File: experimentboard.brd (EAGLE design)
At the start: 105.4 x 100 mm, 72 parts, among them IC1 TL072P, IC2 LM317, IC3 LM337, Q1 27 MHz, U1 PCM1690, U2 PLL1706

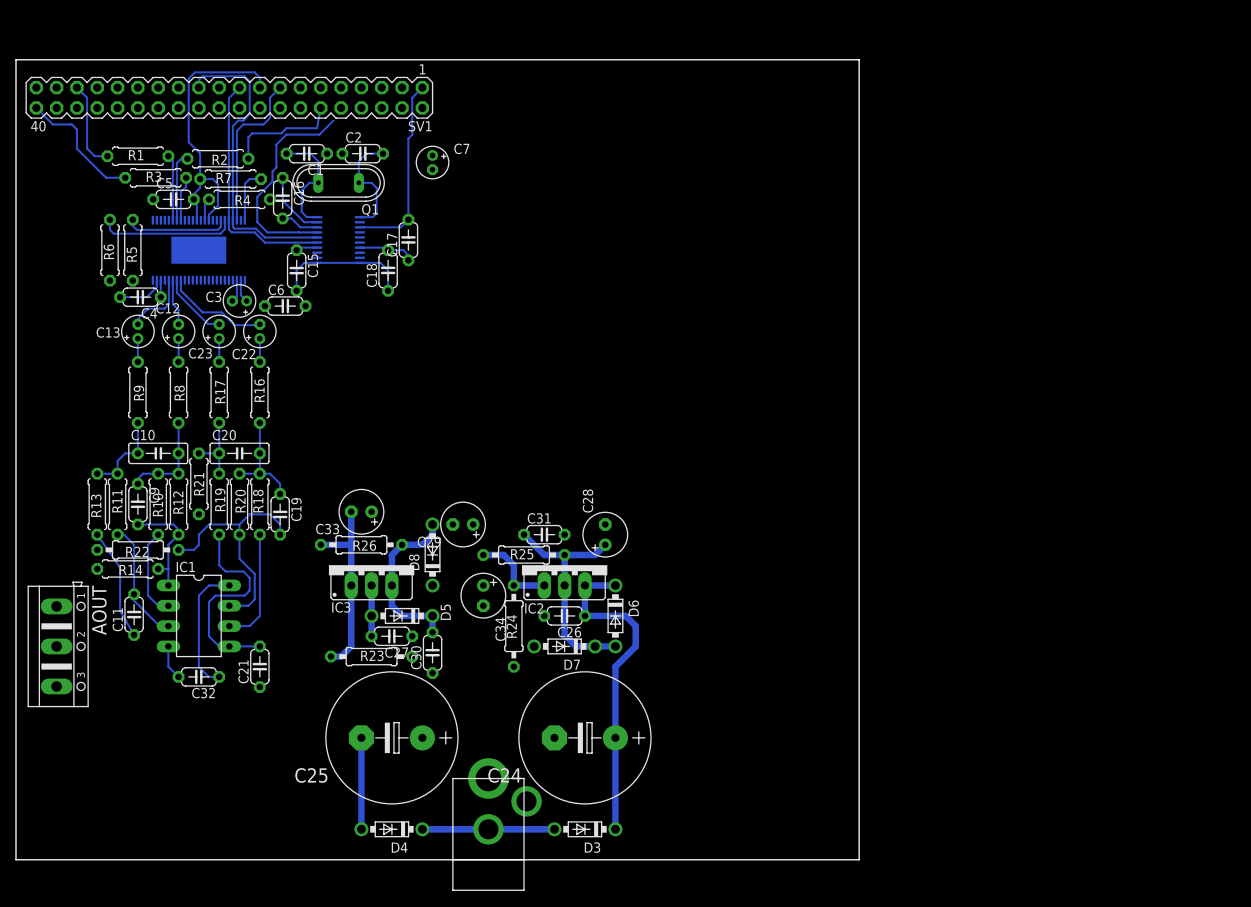
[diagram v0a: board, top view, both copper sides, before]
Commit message: Taking the Beaglebone approach
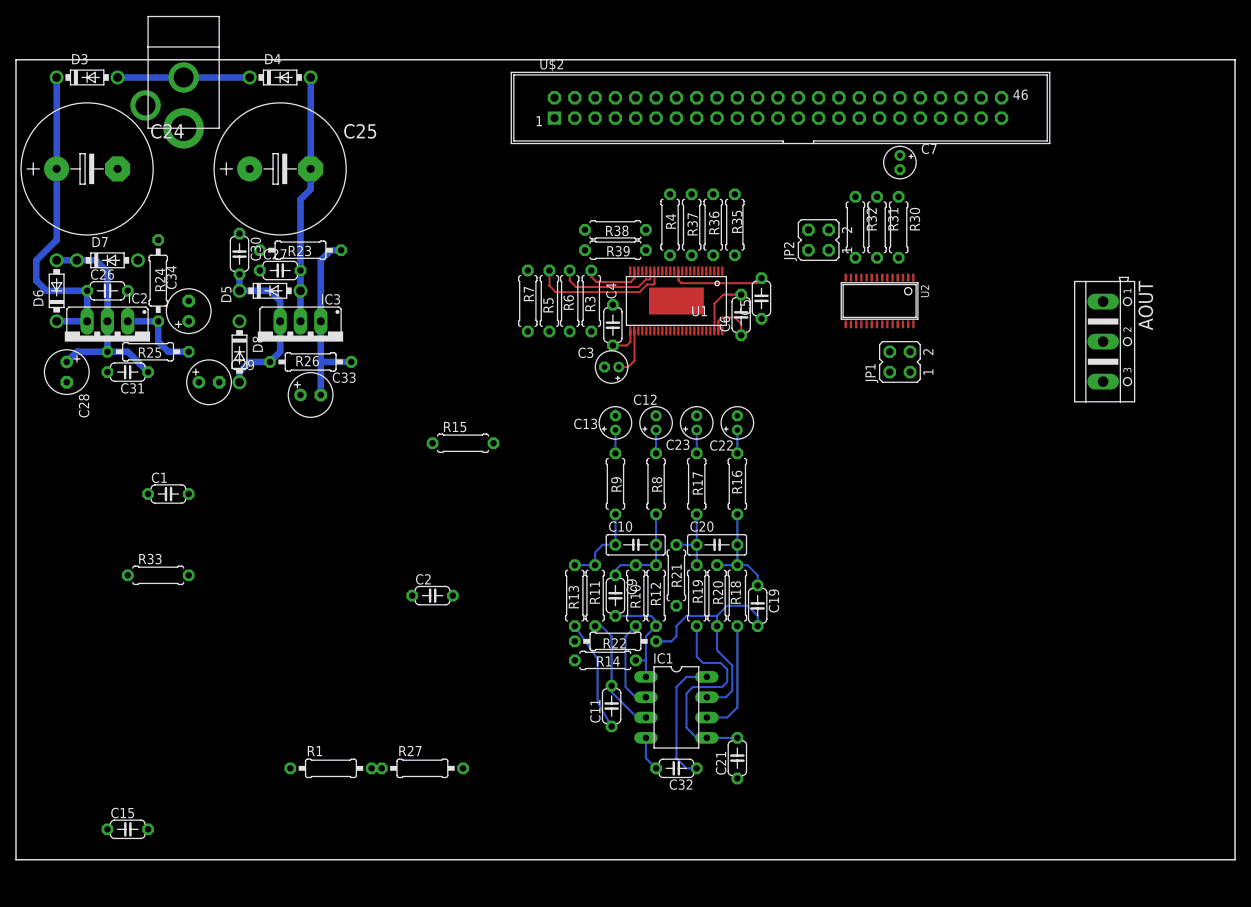
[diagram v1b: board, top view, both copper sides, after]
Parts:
- removed C16, C17, C18: 100 nF ml, rcl:C050-024X044
- removed Q1: 27 MHz, special:QS
- removed R2: 22, rcl:0207/7
- removed SV1: (no value), 0000halfgaar:MA20-2
- added JP1, JP2: (no value), jumper:JP2Q
- added R15: 680, rcl:0207/7
- added R27: 0, rcl:0207/10
- added R30, R31, R32, R33, R35, R36, R37: 22, rcl:0207/7
- added R38, R39: 5.6k, rcl:0207/7
- added U$2: BEAGLEBONEP9, 0000halfgaar:HEADERS23-2
- C1: value 22pf -> 4.7n
- C15: value 100 nF ml -> 1µF ml
- C2: value 22pf -> 68n
- R1: value 22 -> 0; device rcl:0207/7 -> rcl:0207/10
- R23, R24: value 2.7k -> 715
- R3: value 22 -> 10k
- U2: value PLL1706 -> DIR9001; device 0000halfgaar:SSOP20 -> 0000halfgaar:TSSOP28
- moved AOUT 136.2 mm to (135.9, 64.8)
- moved AC 118.9 mm to (16.5, 105.4), turned to 0 degrees
- moved D3 112.7 mm to (8.89, 97.8), turned to 0 degrees
- moved D4 95.0 mm to (33.0, 97.8), turned to 0 degrees
- moved C24 94.5 mm to (8.89, 86.4), turned to 0 degrees
- moved D6 80.8 mm to (5.08, 71.1), turned to 90 degrees
- moved R1 80.2 mm to (39.4, 11.4)
- moved D7 74.8 mm to (11.4, 74.9), turned to 0 degrees
- moved C5 74.5 mm to (93.2, 70.2), turned to 90 degrees
- moved C15 73.0 mm to (14.0, 3.81), turned to 0 degrees
- moved C25 72.5 mm to (33.0, 86.4), turned to 0 degrees
- moved C28 70.3 mm to (6.35, 61.0), turned to 270 degrees
- moved C26 70.1 mm to (11.4, 71.1), turned to 0 degrees
- moved U2 68.1 mm to (108.0, 69.8), flipped to the top, turned to 180 degrees
- moved IC2 63.6 mm to (11.4, 64.8), turned to 180 degrees
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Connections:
- removed net MOSI: SV1.19, U1.20, U2.5
- removed net N$10: R1.1, SV1.35
- removed net N$9: R2.1, SV1.12
- removed net SCKL: SV1.23, U1.21, U2.6
- removed net U1SEL: SV1.15, U1.22
- removed net U2SEL: SV1.10, U2.7
- new net ACLKR: R31.1, U$2.12
- new net ACLKX: R36.1, U$2.31
- new net AHCLKX: R35.1, U$2.29
- new net DIN: R32.1, U$2.32
- new net DIR_AUDIO: U$2.16, U2.1
- new net DOUT: R37.1, U$2.28
- new net FSR: R30.1, U$2.27
- new net MCLK: R4.1, U$2.25
- new net N$20: U2.20
- new net N$51: R32.2, U2.12
- new net N$52: R31.2, U2.11
- new net N$53: R30.2, U2.10
- new net N$54: R33.2, U2.4
- new net N$61: R37.2, U1.8
- new net N$62: R36.2, U1.7
- new net N$63: R35.2, U1.6
- new net RST: U$2.15, U1.15, U2.21
- new net SCL: R38.1, U$2.17, U1.21
- new net SDA: R39.1, U$2.18, U1.20
- net AGND: now also C1.1, C2.1, R1.2, U2.23; no longer C16.1, U2.9
- net DGND: now also C15.2, R1.1, R7.1, U$2.1, U$2.2, U2.19, U2.6, U2.8; no longer C1.1, C15.1, C17.1, C18.2, C2.1, SV1.9, U2.16, U2.17, U2.4
- net N$1: now also JP2.3, U2.14; no longer R1.2, U1.6
- net N$2: now also R3.2, U1.23; no longer R2.2, U1.7
- net N$3: now also JP2.1, U2.13; no longer R3.2, U1.8
- net N$4: now also C1.2, R15.1, U2.22; no longer R4.1, U2.3
- net N$6: now also C2.2, R15.2; no longer C1.2, Q1.2, U2.10
- net N$7: now also JP1.4, U2.25; no longer C2.2, Q1.1, U2.11
- net N$8: now also JP1.2, U2.26; no longer R3.1, SV1.40
- net V+: now also R27.2
- net VCC: now also R27.1, U$2.5, U$2.6, U2.24; no longer C16.2, U2.8
- net VDD: now also C15.1, JP1.1, JP1.3, JP2.2, JP2.4, R3.1, R38.2, R39.2, U$2.3, U$2.4, U2.5; no longer C15.2, C17.2, C18.1, R7.1, SV1.1, SV1.17, U1.15, U2.1, U2.13, U2.20
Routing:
- net VDD: track 78.0 -> 12.0 mm
- net SCKL: track 38.3 -> 0.00 mm
- net MOSI: track 30.0 -> 0.00 mm
- net U2SEL: track 27.1 -> 0.00 mm
- net U1SEL: track 20.3 -> 0.00 mm
- net N$8: track 16.1 -> 0.00 mm
- net N$6: track 14.4 -> 0.00 mm
- net N$9: track 14.3 -> 0.00 mm
- net N$7: track 14.1 -> 0.00 mm
- net N$41: track 17.8 -> 31.0 mm
- net N$36: track 13.0 -> 0.13 mm
- net N$10: track 11.1 -> 0.00 mm
- net DGND: track 9.80 -> 0.00 mm
- net N$35: track 8.51 -> 0.09 mm
- net N$1: track 8.23 -> 0.00 mm
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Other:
- board size 105.4 x 100 mm -> 152.4 x 100 mm
